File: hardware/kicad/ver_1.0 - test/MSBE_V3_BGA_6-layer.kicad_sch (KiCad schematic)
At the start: 85 parts, among them J1 High-V, J2 Low-V, J3 Low-V-TH, J4 Touch Pads, J5 UART, J6 USB, J7 Prog, U1 NPM1100-CAAA-R7, U2 NRF5340-CLAA-R, U3 MPR121QR2, U4 BMA400, U6 MAX98357AEWL_T, Y2 32.768kHz, Y3 32MHz

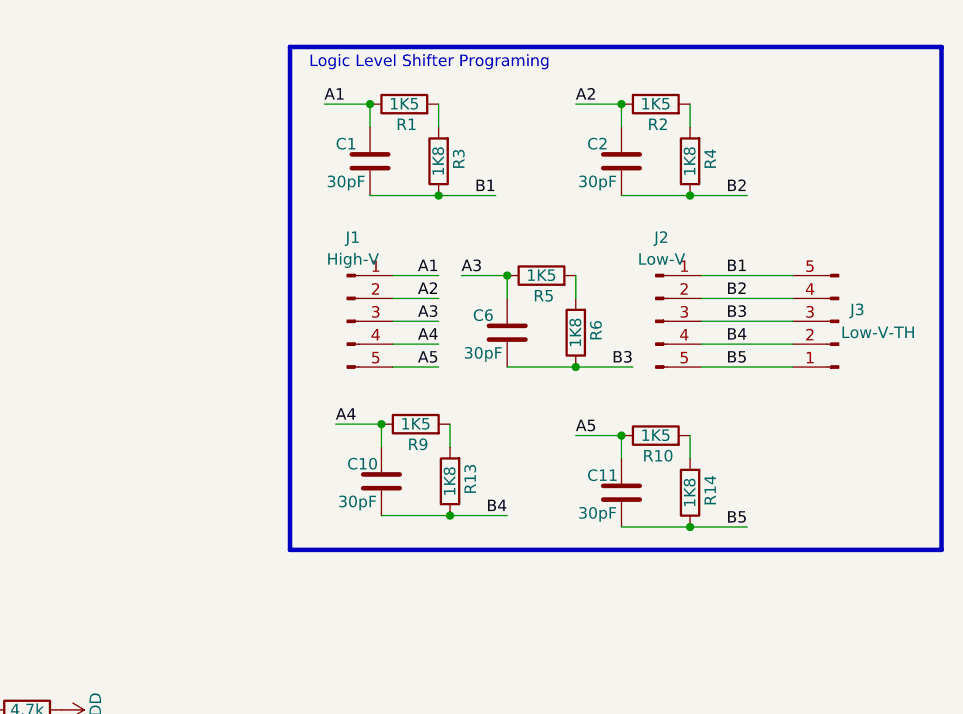
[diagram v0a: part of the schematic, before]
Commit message: added silckscreen
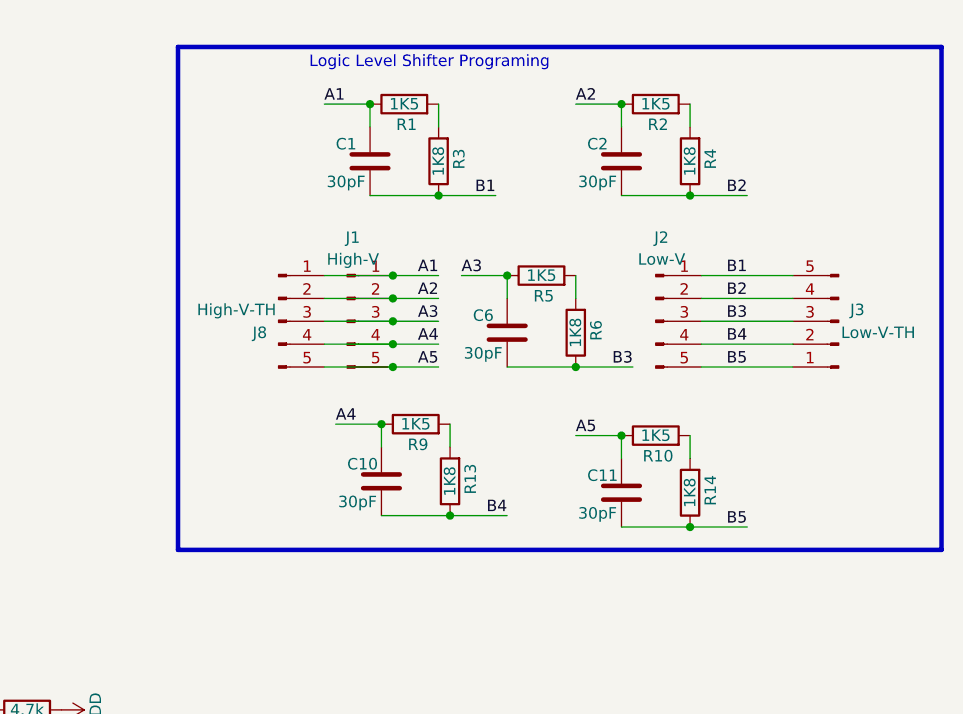
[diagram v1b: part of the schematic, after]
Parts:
- added J8: High-V-TH, Connector_PinHeader_2.54mm:PinHeader_1x05_P2.54mm_Vertical, symbol Connector:Conn_01x05_Pin
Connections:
- net A1: now also J8.1 (Pin_1)
- net A2: now also J8.2 (Pin_2)
- net A3: now also J8.3 (Pin_3)
- net A4: now also J8.4 (Pin_4)
- net A5: now also J8.5 (Pin_5)
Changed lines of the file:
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@@
 	)
 	(rectangle
-		(start 328.93 20.32)
+		(start 316.484 20.32)
 		(end 401.32 76.2)
 		(stroke
@@
 	)
 	(junction
+		(at 340.36 50.8)
+		(diameter 0)
+		(color 0 0 0 0)
+	)
+	(junction
 		(at 339.09 62.23)
 		(diameter 0)
@@
 	)
 	(junction
+		(at 340.36 45.72)
+		(diameter 0)
+		(color 0 0 0 0)
+	)
+	(junction
 		(at 273.05 106.68)
 		(diameter 0)
@@
 	)
 	(junction
+		(at 340.36 48.26)
+		(diameter 0)
+		(color 0 0 0 0)
+	)
+	(junction
 		(at 285.75 129.54)
 		(diameter 0)
@@
 	)
 	(junction
+		(at 340.36 53.34)
+		(diameter 0)
+		(color 0 0 0 0)
+	)
+	(junction
 		(at 99.695 254)
 		(diameter 0)
@@
 	)
 	(junction
+		(at 340.36 55.88)
+		(diameter 0)
+		(color 0 0 0 0)
+	)
+	(junction
 		(at 105.41 66.04)
 		(diameter 0)
@@
 	(wire
 		(pts
+			(xy 332.74 53.34) (xy 340.36 53.34)
+		)
+		(stroke
+			(width 0)
+			(type default)
+		)
+	)
+	(wire
+		(pts
 			(xy 274.32 124.46) (xy 274.32 127)
 		)
@@
 	(wire
 		(pts
+			(xy 332.74 48.26) (xy 340.36 48.26)
+		)
+		(stroke
+			(width 0)
+			(type default)
+		)
+	)
+	(wire
+		(pts
 			(xy 138.43 121.92) (xy 140.97 121.92)
 		)
@@
 	(wire
 		(pts
+			(xy 332.74 45.72) (xy 340.36 45.72)
+		)
+		(stroke
+			(width 0)
+			(type default)
+		)
+	)
+	(wire
+		(pts
 			(xy 163.83 99.06) (xy 176.53 99.06)
 		)
@@
 	(wire
 		(pts
+			(xy 332.74 50.8) (xy 340.36 50.8)
+		)
+		(stroke
+			(width 0)
+			(type default)
+		)
+	)
+	(wire
+		(pts
 			(xy 172.72 73.66) (xy 175.26 73.66)
 		)
@@
 	(wire
 		(pts
+			(xy 332.74 55.88) (xy 340.36 55.88)
+		)
+		(stroke
+			(width 0)
+			(type default)
+		)
+	)
+	(wire
+		(pts
 			(xy 105.41 58.42) (xy 105.41 59.69)
 		)
@@
 					(unit 1)
 				)
+			)
+		)
+	)
+	(symbol
+		(lib_id "Connector:Conn_01x05_Pin")
+		(at 327.66 50.8 0)
+		(unit 1)
+		(exclude_from_sim no)
+		(in_bom yes)
+		(on_board yes)
+		(dnp no)
+		(property "Reference" "J8"
+			(at 326.39 52.0701 0)
+			(effects
+				(font
+					(size 1.27 1.27)
+				)
+				(justify right)
+			)
+		)
+		(property "Value" "High-V-TH"
+			(at 327.406 49.53 0)
+			(effects
+				(font
+					(size 1.27 1.27)
+				)
+				(justify right)
+			)
+		)
+		(property "Footprint" "Connector_PinHeader_2.54mm:PinHeader_1x05_P2.54mm_Vertical"
+			(at 327.66 50.8 0)
+			(effects
+				(font
+					(size 1.27 1.27)
+				)
+				(hide yes)
+			)
+		)
+		(property "Datasheet" "~"
+			(at 327.66 50.8 0)
+			(effects
+				(font
+					(size 1.27 1.27)
+				)
+				(hide yes)
+			)
+		)
+		(property "Description" "Generic connector, single row, 01x05, script generated"
+			(at 327.66 50.8 0)
+			(effects
+				(font
+					(size 1.27 1.27)
+				)
+				(hide yes)
+			)
+		)
+		(pin "2"
+		)
+		(pin "1"
+		)
+		(pin "3"
+		)
+		(pin "5"
+		)
+		(pin "4"
+		)
+		(instances
+			(project "MSBE_V3_BGA_6-layer"
+				(path "/7e9bed8c-661c-41cb-9879-cab5c0a53fc4"
+					(reference "J8")
+					(unit 1)
+				)
